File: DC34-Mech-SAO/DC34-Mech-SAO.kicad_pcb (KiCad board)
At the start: 2 copper layers, 27.9 x 38 mm, 20 parts, among them J1 Conn_01x06_Male, J2 Conn_01x03_Male, U1 ATtiny816-M

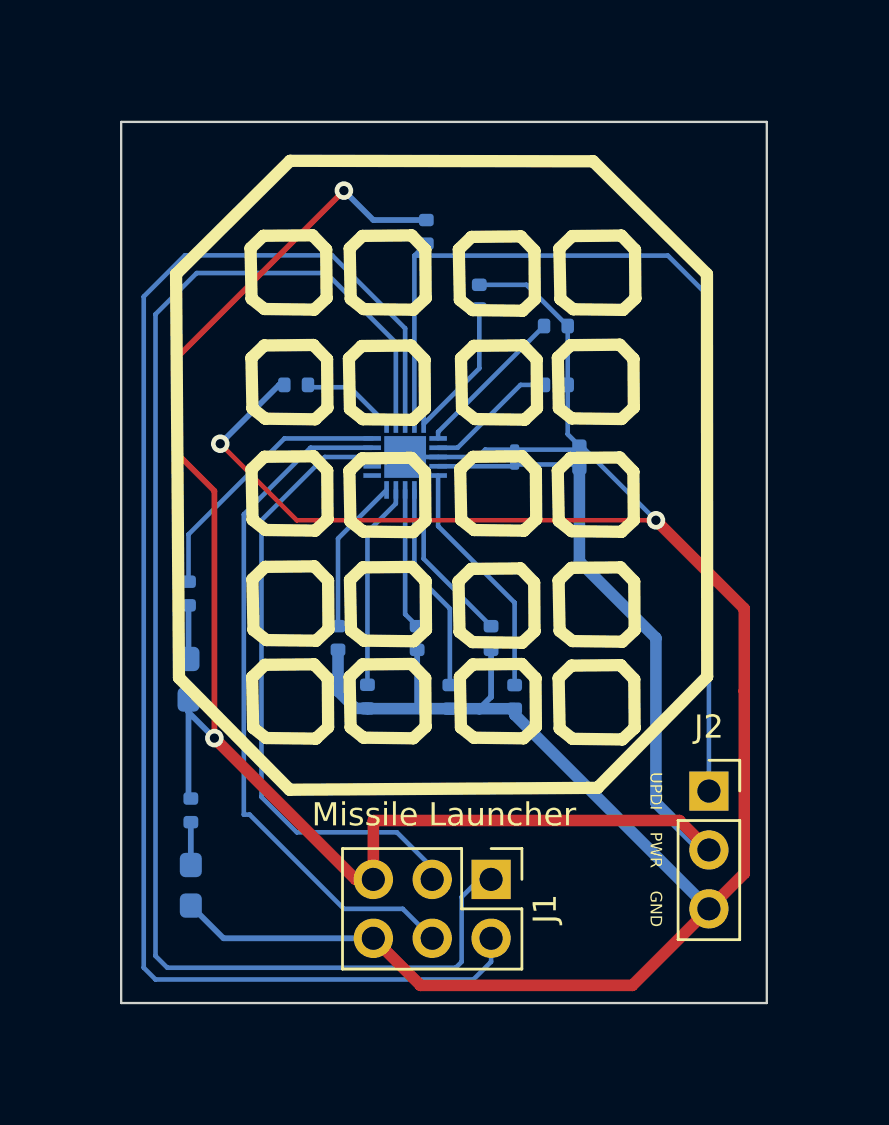
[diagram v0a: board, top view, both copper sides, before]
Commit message: Updates to project over last few days.
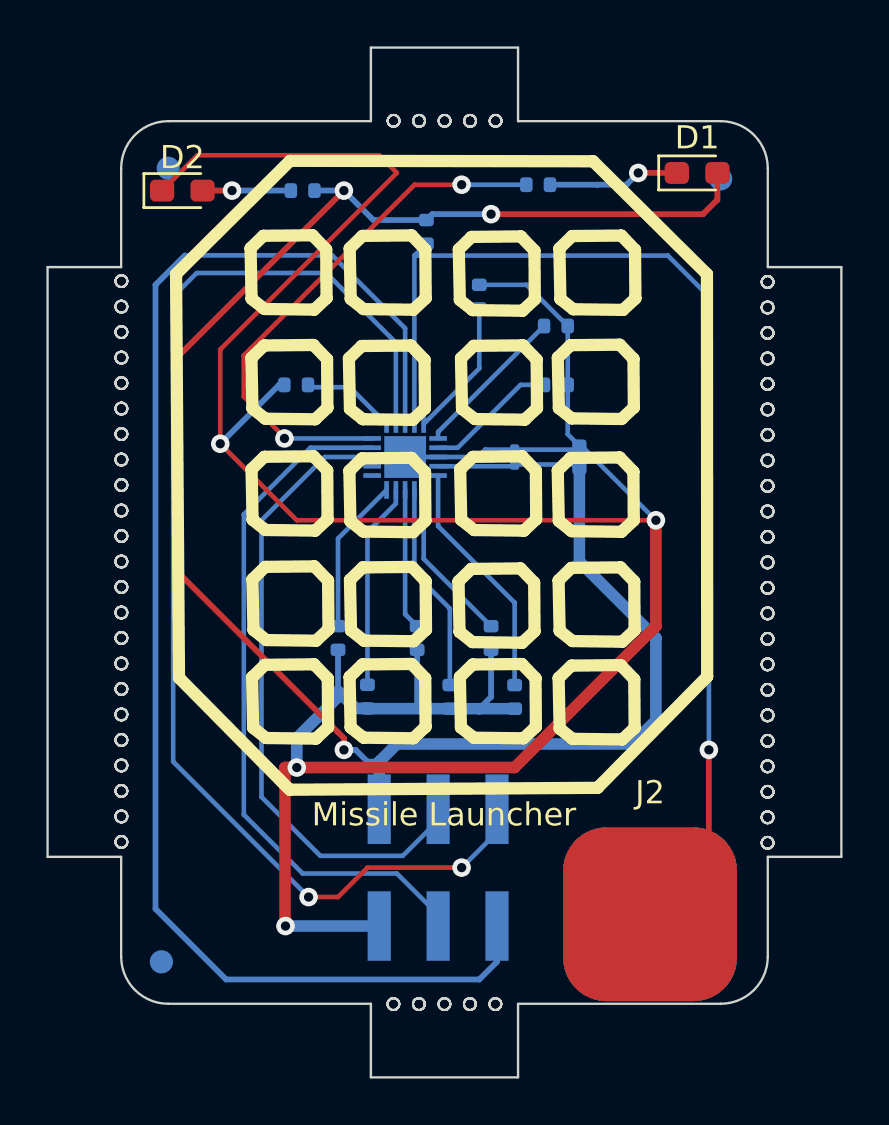
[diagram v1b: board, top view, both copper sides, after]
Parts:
- added REF**: Fiducial_1mm_Mask2mm, Fiducial:Fiducial_1mm_Mask2mm, B.Cu at (156.7, 64.5)
- added REF**: Fiducial_1mm_Mask2mm, Fiducial:Fiducial_1mm_Mask2mm, B.Cu at (132.6, 98.3)
- added REF**: Fiducial_1mm_Mask2mm, Fiducial:Fiducial_1mm_Mask2mm, B.Cu at (132.9, 64.1)
- D1, D2: moved to F.Cu
- J1: footprint Connector_PinHeader_2.54mm:PinHeader_2x03_P2.54mm_Vertical -> Connector_PinSocket_2.54mm:PinSocket_2x03_P2.54mm_Vertical_SMD; moved to B.Cu
- J2: value Conn_01x03_Male -> Conn_01x01_Male; footprint Connector_PinSocket_2.54mm:PinSocket_1x03_P2.54mm_Vertical -> UPDI_ICRP:Aligator_TIP
- R1: value 10k -> 2k
- moved D1 31.0 mm to (155.7, 64.3), turned to 0 degrees
- moved D2 30.0 mm to (133.5, 65.0), turned to 0 degrees
- moved R2 27.2 mm to (138.7, 65.0), turned to 180 degrees
- moved R1 23.2 mm to (148.8, 64.8), turned to 180 degrees
- moved J2 4.79 mm to (153.7, 95.0)
- moved J1 2.34 mm to (144.5, 94.2), turned to 90 degrees
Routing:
- net UPDI: track 42.8 -> 57.5 mm, vias 0 -> 1
- net Net-(R1-Pad2): track 11.7 -> 23.3 mm, vias 0 -> 2
- net GND: track 117.5 -> 125.7 mm, vias 2 -> 4
- net GPIO1: track 61.5 -> 53.4 mm, vias 0 -> 2
- net PWR: track 89.8 -> 84.4 mm, vias 1 -> 3
- net Net-(D1-Pad1): track 2.31 -> 5.69 mm, vias 0 -> 1
- net Net-(D2-Pad2): track 1.85 -> 3.81 mm, vias 0 -> 1
- net GPIO2: track 62.9 -> 61.5 mm
- net SDA: track 27.0 -> 27.6 mm
- net (no net): vias 1 -> 0
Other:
- board size 27.9 x 38 mm -> 34.2 x 44.4 mm
- board text added: "Mech Fighters SAO Rev 3"
- board text removed: "Mech Fighters SAO Rev 1"
